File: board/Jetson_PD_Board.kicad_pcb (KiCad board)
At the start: 2 copper layers, 47 parts, among them J1 USB4081-03-A, J2 768250002, Q1 NTTFS5C673NLTAG, Q2 NTTFS5C673NLTAG, Q3 NTTFS5C673NLTAG, U1 APK43070DKZ-13-FA01, U2 USBLC6-2SC6

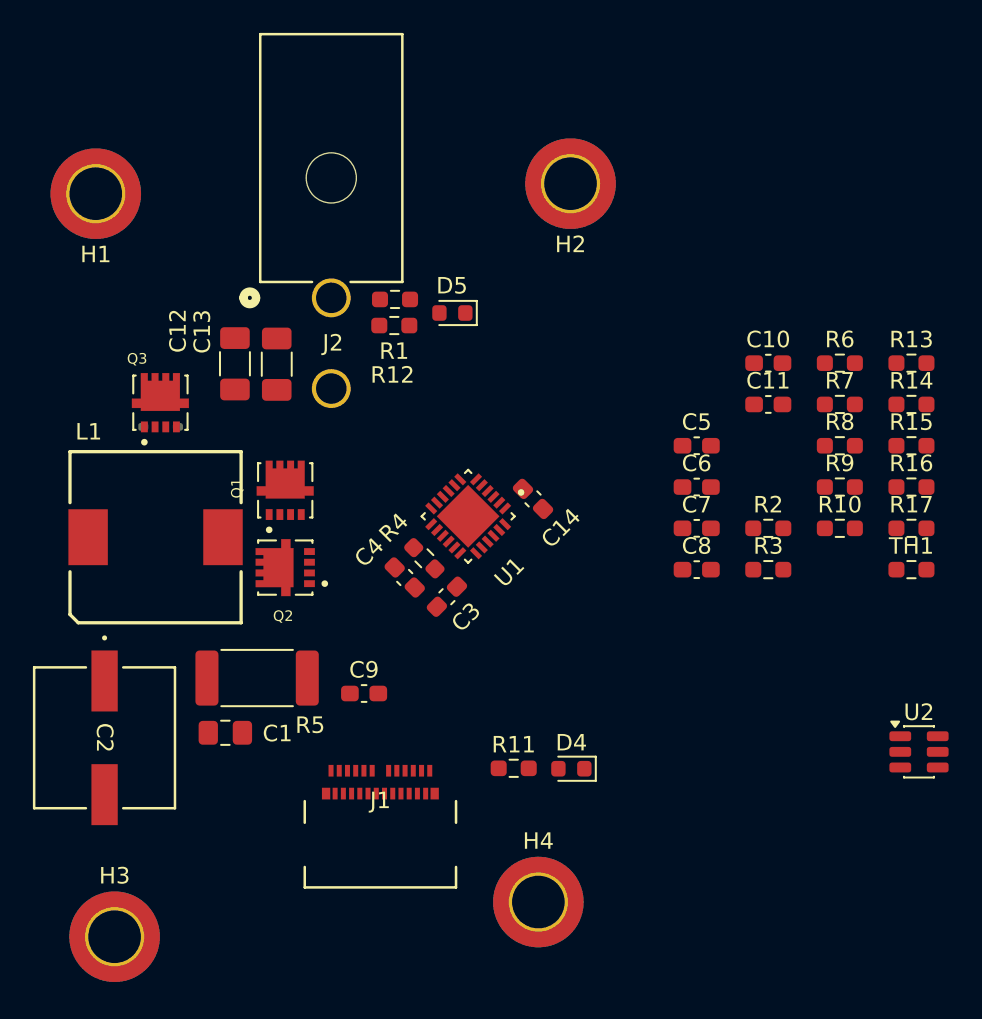
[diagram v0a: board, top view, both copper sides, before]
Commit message: Worked on layout
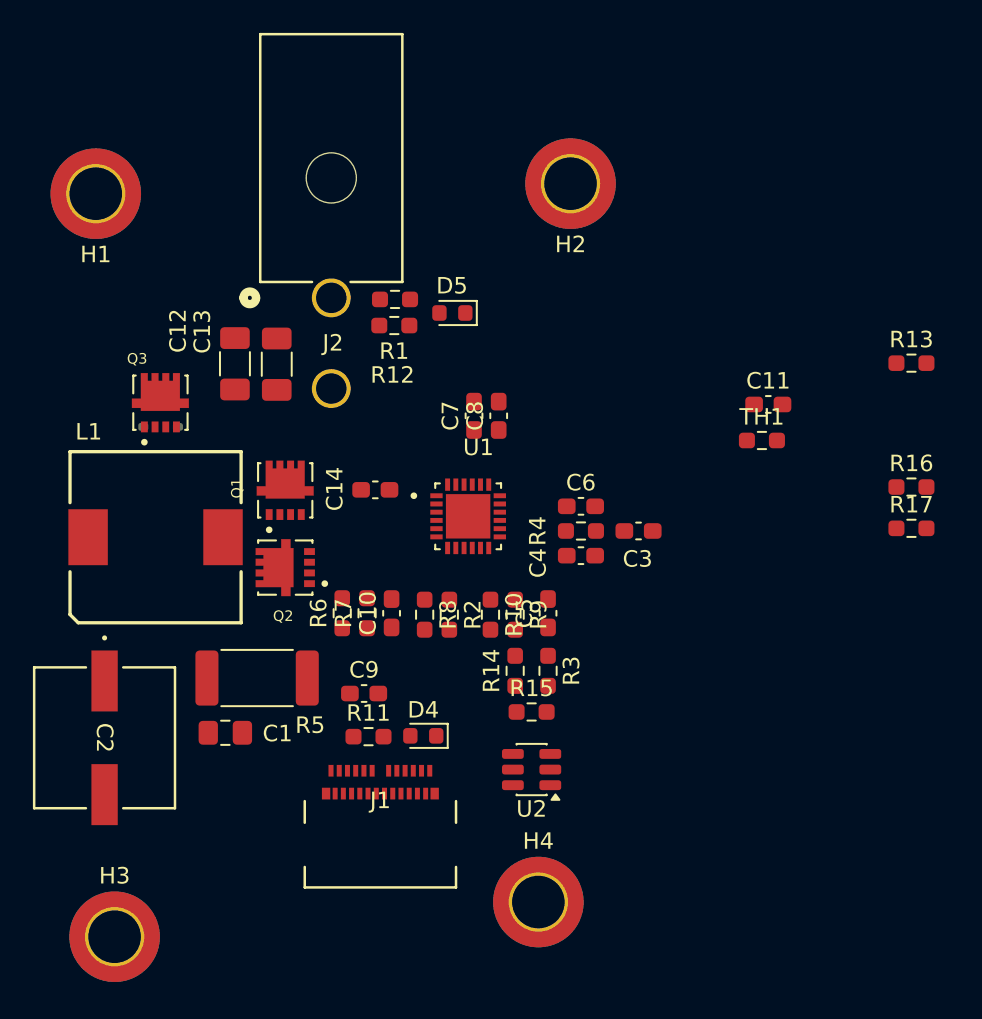
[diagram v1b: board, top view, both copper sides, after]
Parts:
- moved R6 33.9 mm to (128.5, 98.5), turned to 90 degrees
- moved R7 31.4 mm to (130.0, 98.5), turned to 90 degrees
- moved R14 29.0 mm to (139.0, 102.0), turned to 90 degrees
- moved R15 28.2 mm to (140.0, 104.5)
- moved C10 27.5 mm to (131.5, 98.5), turned to 90 degrees
- moved R8 27.2 mm to (133.5, 98.6), turned to -90 degrees
- moved U2 23.6 mm to (140.0, 108.0), turned to 180 degrees
- moved R10 21.9 mm to (137.5, 98.6), turned to -90 degrees
- moved R9 21.2 mm to (139.0, 98.6), turned to -90 degrees
- moved R2 20.1 mm to (135.0, 98.6), turned to -90 degrees
- moved C8 15.2 mm to (138.0, 86.5), turned to 90 degrees
- moved C7 15.2 mm to (136.5, 86.5), turned to 90 degrees
- moved R3 14.7 mm to (141.0, 102.0), turned to -90 degrees
- moved C5 13.6 mm to (141.0, 98.5), turned to 90 degrees
- moved C3 12.3 mm to (146.5, 93.5), turned to 0 degrees
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
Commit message: Placed most components
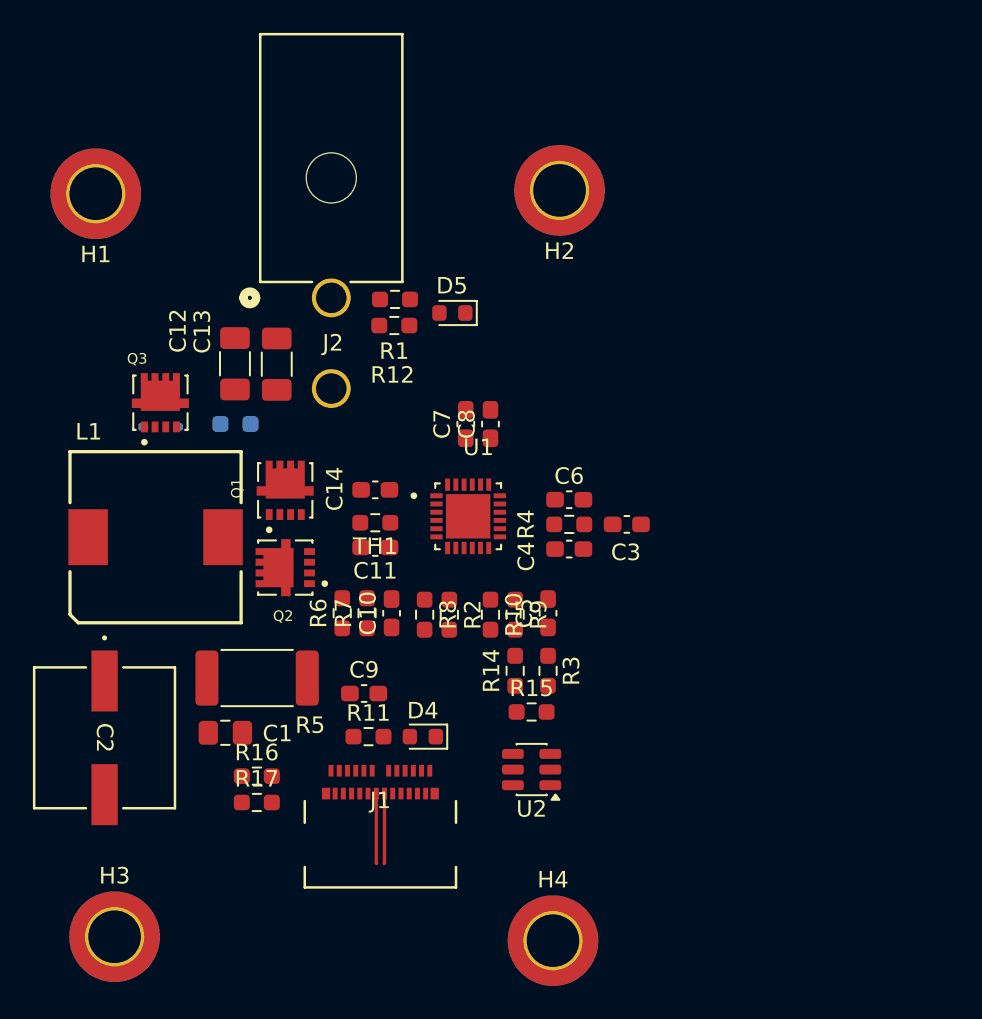
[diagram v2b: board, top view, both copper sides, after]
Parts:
- R13: moved to B.Cu
- moved R16 43.5 mm to (123.3, 108.4)
- moved R17 43.1 mm to (123.3, 110.0)
- moved R13 41.3 mm to (122.0, 87.0)
- moved C11 25.4 mm to (130.5, 94.5), turned to 180 degrees
- moved TH1 24.0 mm to (130.5, 93.0), turned to 180 degrees
- moved H4 2.51 mm to (141.3, 118.4)
- moved C3 0.82 mm to (145.8, 93.1)
- moved C4 0.82 mm to (142.3, 94.6)
- moved C6 0.82 mm to (142.3, 91.6)
- moved R4 0.82 mm to (142.3, 93.1)
- moved H2 0.78 mm to (141.7, 72.8)
- moved C7 0.71 mm to (136.0, 87.0)
- moved C8 0.71 mm to (137.5, 87.0)
- moved D4 0.06 mm to (133.4, 106.0)
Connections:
- net Net-(J1-DN2) renamed /USB_DN
- net Net-(J1-DP2) renamed /USB_DP
- net Net-(R14-Pad2) renamed /DP
- net Net-(R15-Pad2) renamed /DN
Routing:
- net /USB_DP: track 0.00 -> 4.25 mm
- net /USB_DN: track 0.00 -> 4.25 mm
